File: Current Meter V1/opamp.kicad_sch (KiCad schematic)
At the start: 14 parts, among them U503 MCP6002-xSN

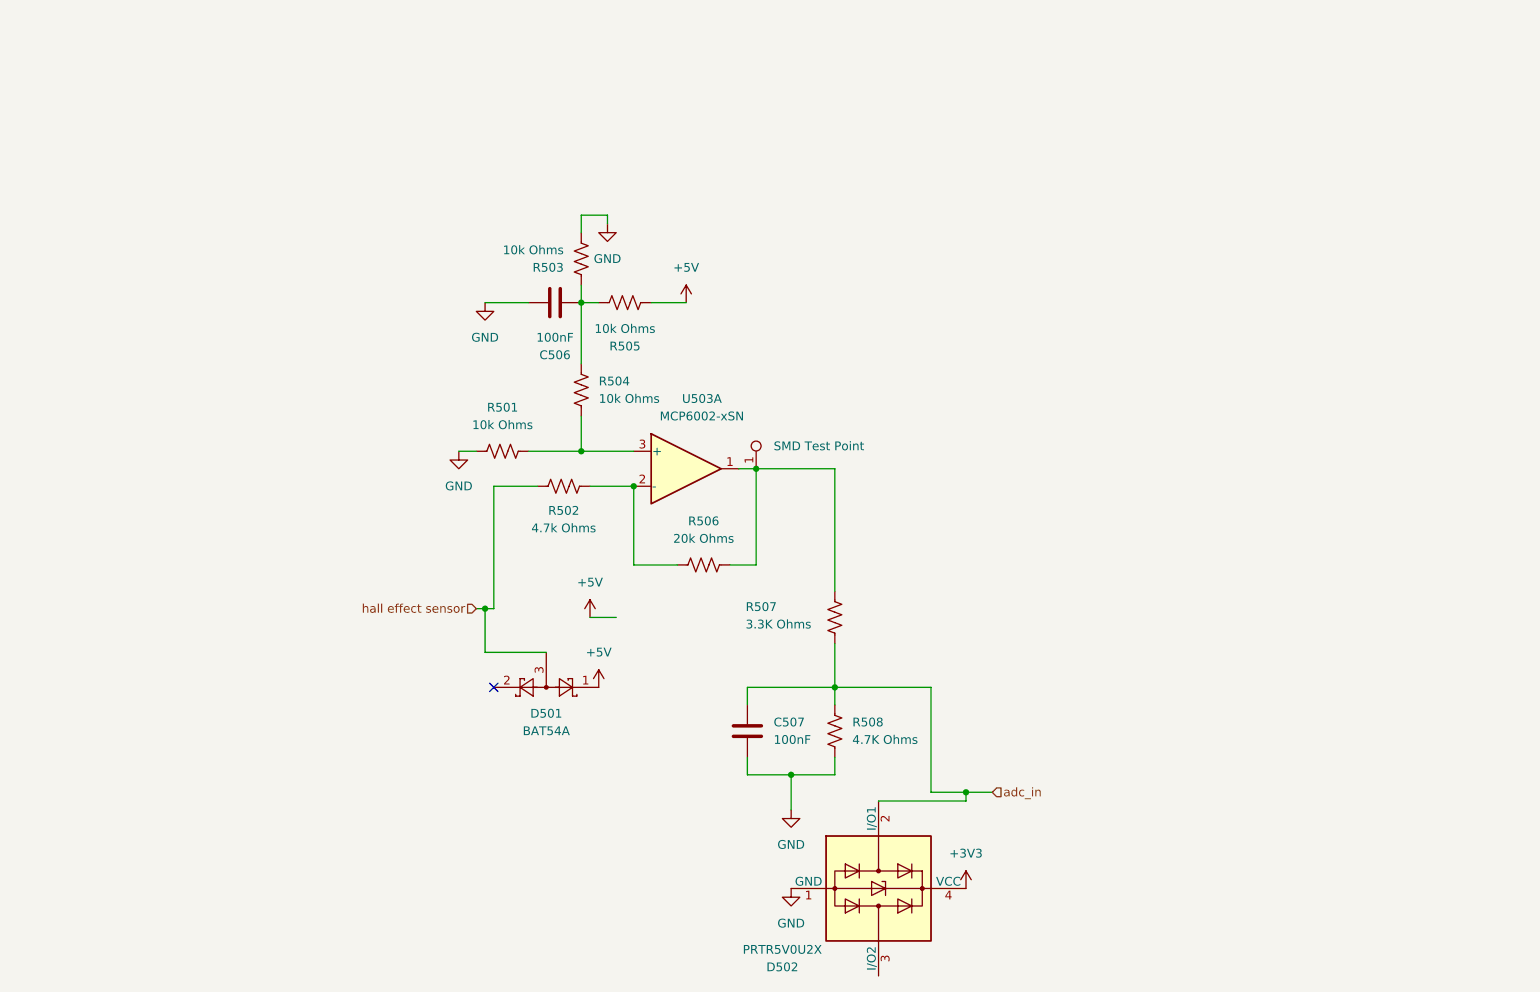
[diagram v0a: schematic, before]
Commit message: microcontroller update
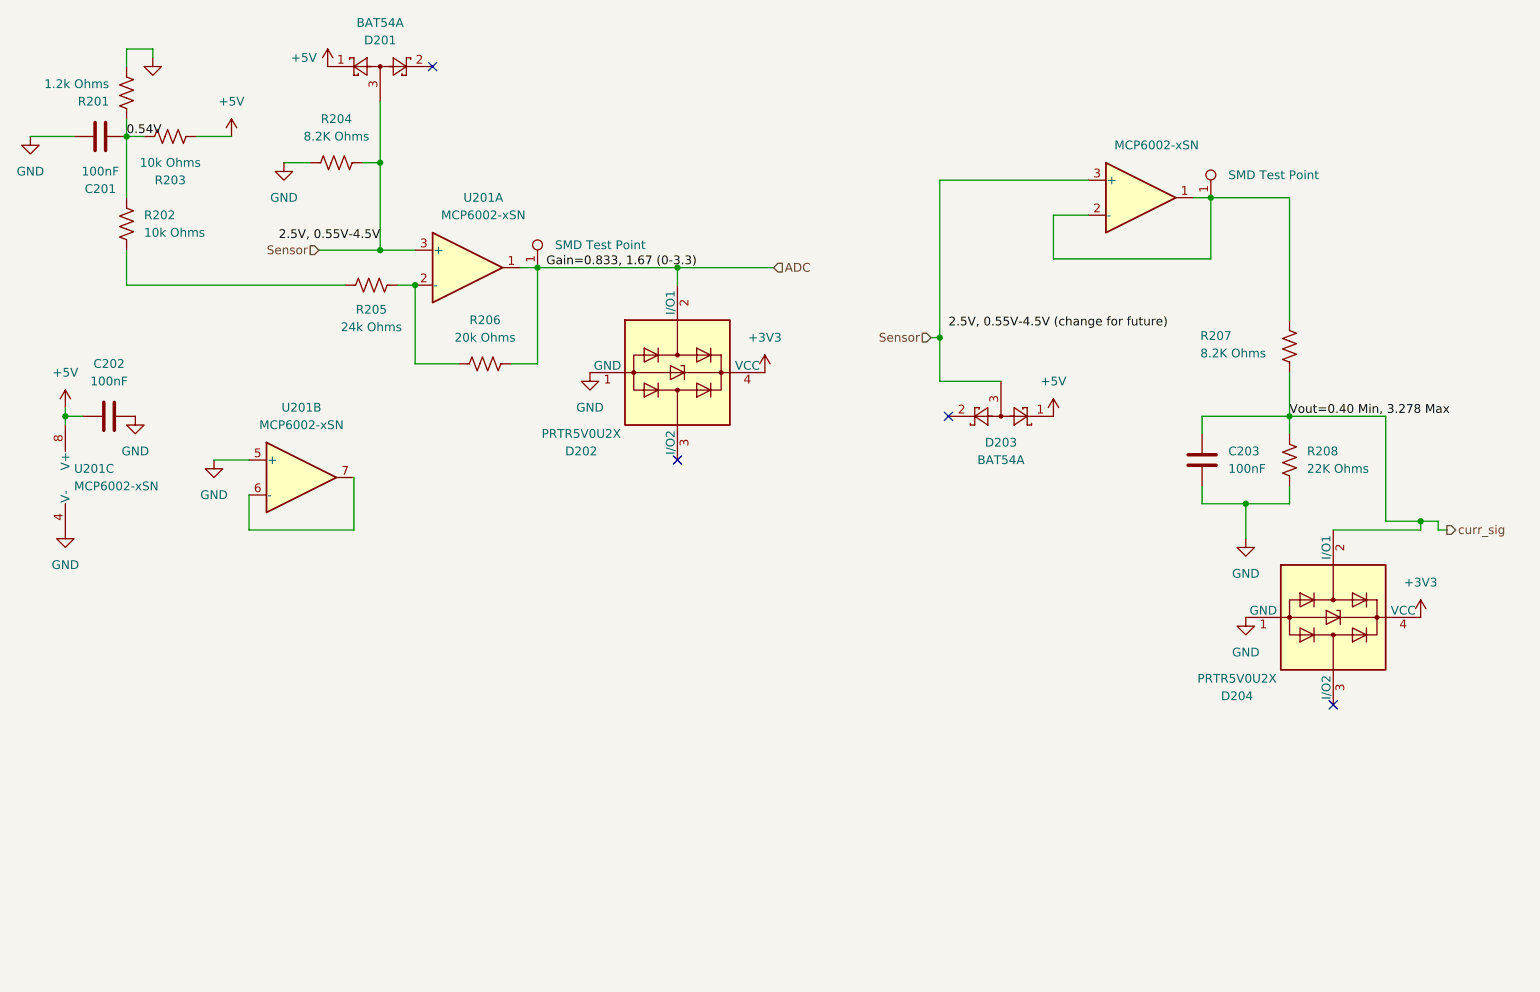
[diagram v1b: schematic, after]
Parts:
- removed C506, C507: 100nF, symbol Device:C
- removed D501: BAT54A, Package_TO_SOT_SMD:SOT-23, symbol Diode:BAT54A
- removed D502: PRTR5V0U2X, Package_TO_SOT_SMD:SOT-143, symbol Power_Protection:PRTR5V0U2X
- removed R501, R503, R504, R505: 10k Ohms, symbol Device:R_US
- removed R502: 4.7k Ohms, symbol Device:R_US
- removed R506: 20k Ohms, symbol Device:R_US
- removed R507: 3.3K Ohms, symbol Device:R_US
- removed R508: 4.7K Ohms, symbol Device:R_US
- removed TP501: SMD Test Point, TestPoint:TestPoint_Keystone_5019_Miniature, symbol bfr_utilities:SMD_Test_Point
- removed U503: MCP6002-xSN, symbol Amplifier_Operational:MCP6002-xSN
- added C201, C202, C203: 100nF, symbol Device:C
- added D201, D203: BAT54A, Package_TO_SOT_SMD:SOT-23, symbol Diode:BAT54A
- added D202, D204: PRTR5V0U2X, Package_TO_SOT_SMD:SOT-143, symbol Power_Protection:PRTR5V0U2X
- added R201: 1.2k Ohms, symbol Device:R_US
- added R202, R203: 10k Ohms, symbol Device:R_US
- added R204, R207: 8.2K Ohms, symbol Device:R_US
- added R205: 24k Ohms, symbol Device:R_US
- added R206: 20k Ohms, symbol Device:R_US
- added R208: 22K Ohms, symbol Device:R_US
- added TP201, TP202: SMD Test Point, TestPoint:TestPoint_Keystone_5019_Miniature, symbol bfr_utilities:SMD_Test_Point
- added U201, U202: MCP6002-xSN, symbol Amplifier_Operational:MCP6002-xSN
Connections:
- net +3V3: now also D202.4 (VCC), D204.4 (VCC)
- net +5V: now also C202.1, D201.1, D203.1, R203.1, U201.8 (V+)
- net GND: now also C201.2, C202.2, C203.2, D202.1 (GND), D204.1 (GND), R201.2, R204.1, R208.2, U201.4 (V-), U201.5 (+)
- new net: R205.2, R206.1, U201.2 (-)
- new net: R207.1, TP202.1, U202.1, U202.2 (-)
- new net: R202.2, R205.1
- new net: U201.6 (-), U201.7
- new net 0.54V: C201.1, R201.1, R202.1, R203.2
- new net ADC: D202.2 (I/O1), R206.2, TP201.1, U201.1
- new net Sensor: D201.3, D203.3, R204.2, U201.3 (+), U202.3 (+)
- new net curr_sig: C203.1, D204.2 (I/O1), R207.2, R208.1
- no-connect marks 1 -> 4
